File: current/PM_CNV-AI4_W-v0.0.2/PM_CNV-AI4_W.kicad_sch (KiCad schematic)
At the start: 77 parts, among them J1 AFA07-S12FCC-00, J10 FFC_10P_P1.0_50mm_reverse, J2 AFA07-S12FCC-00, J3 15EDGRHC-THR-3.5-14P, J4 15EDGRHC-THR-3.5-14P, J5 AFA07-S12FCC-00, J50 FFC_12P_P1.0_100mm_straight, J8 15EDGKNH-3.5-14P, J9 15EDGKNH-3.5-14P, U2 5117, U3 5117, U4 CA-IS3105W, U5 CA-IS3741HW, U6 SN74LVC2G14DBVR, U7 AD7193BRUZ

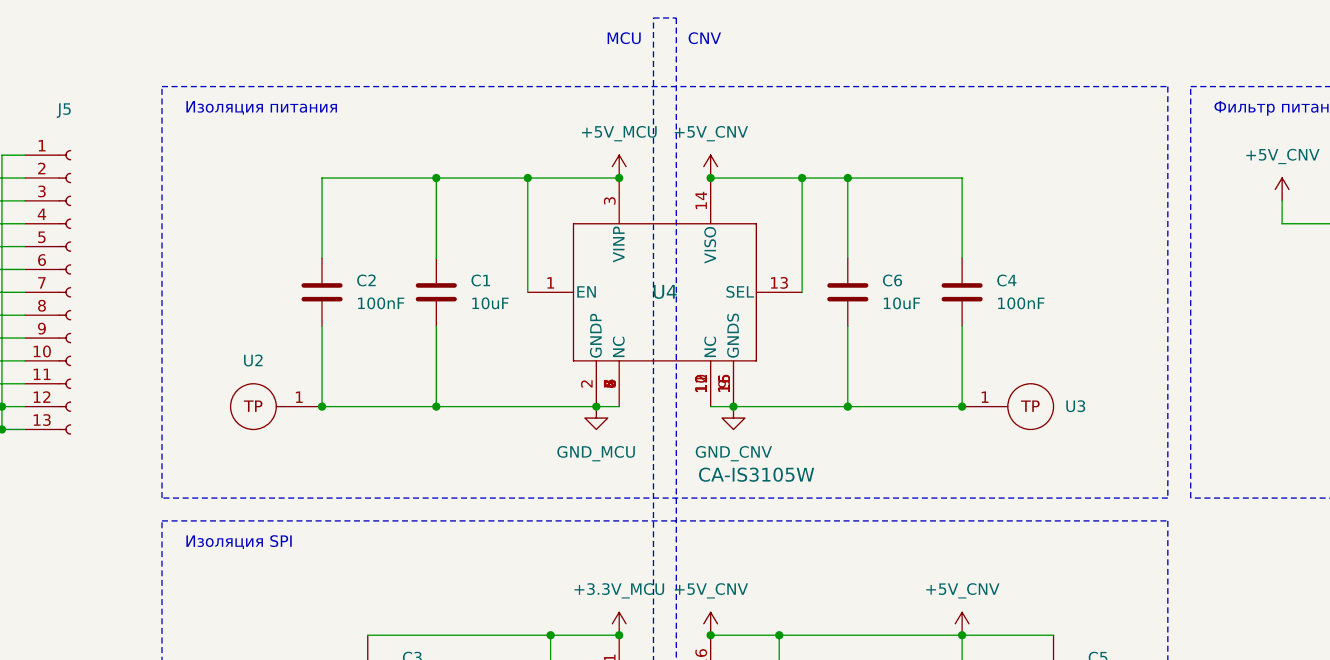
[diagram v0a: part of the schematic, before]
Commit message: update
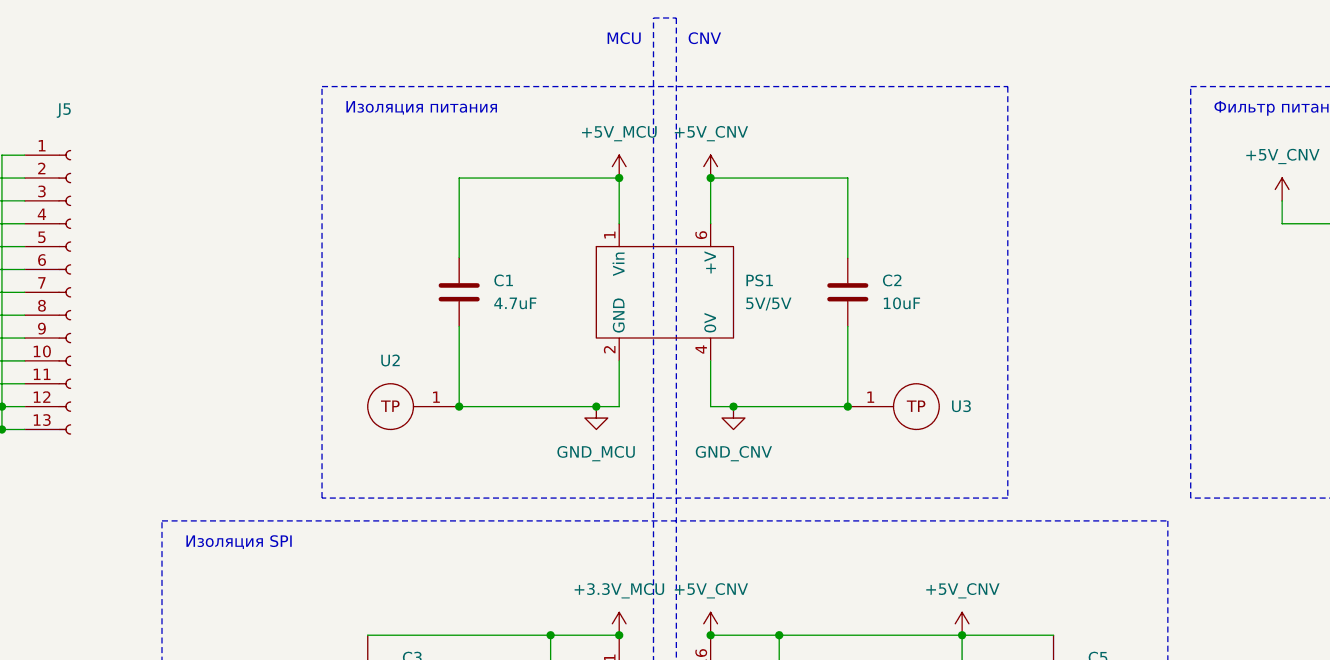
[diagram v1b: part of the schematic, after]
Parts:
- removed C1, C6: 10uF, Capacitor_SMD:C_0805_2012Metric, symbol kicad_inventree_lib:C_10uF_16V_0805_MLCC-X7R
- removed C2, C4: 100nF, Capacitor_SMD:C_0603_1608Metric, symbol kicad_inventree_lib:C_100nF_16V_0603_MLCC-X7R
- removed U4: CA-IS3105W, kicad_inventree_lib:SOIC16-WBW_CLG-M, symbol kicad_inventree_lib:CA-IS3105W
- added C1: 4.7uF, Capacitor_SMD:C_0805_2012Metric, symbol kicad_inventree_lib: C_4.7uF_16V_0805_MLCC-X7R
- added C2: 10uF, Capacitor_SMD:C_0805_2012Metric, symbol kicad_inventree_lib:C_10uF_16V_0805_MLCC-X7R
- added PS1: 5V/5V, kicad_inventree_lib:B2405LS-1WR3, symbol kicad_inventree_lib:B0505LS-1W
- JP1, JP2, JP3, JP4: footprint Jumper:SolderJumper-2_P1.3mm_Open_RoundedPad1.0x1.5mm -> kicad_inventree_lib:SolderJumper-2_P1.3mm_Open_RoundedPad1.0x1.5mm; symbol Jumper:SolderJumper_2_Open -> kicad_inventree_lib:SolderJumper_2_Open
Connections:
- net +5V_CNV: now also C2.1, PS1.6 (+V)
- net +5V_MCU: now also C1.1, PS1.1 (Vin)
- net GND_CNV: now also C2.2, PS1.4 (0V)
- net GND_MCU: now also C1.2, PS1.2 (GND)
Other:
- moved on the sheet: U2, U3
